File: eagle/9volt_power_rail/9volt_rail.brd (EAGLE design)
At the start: 96.2 x 63.2 mm, 22 parts

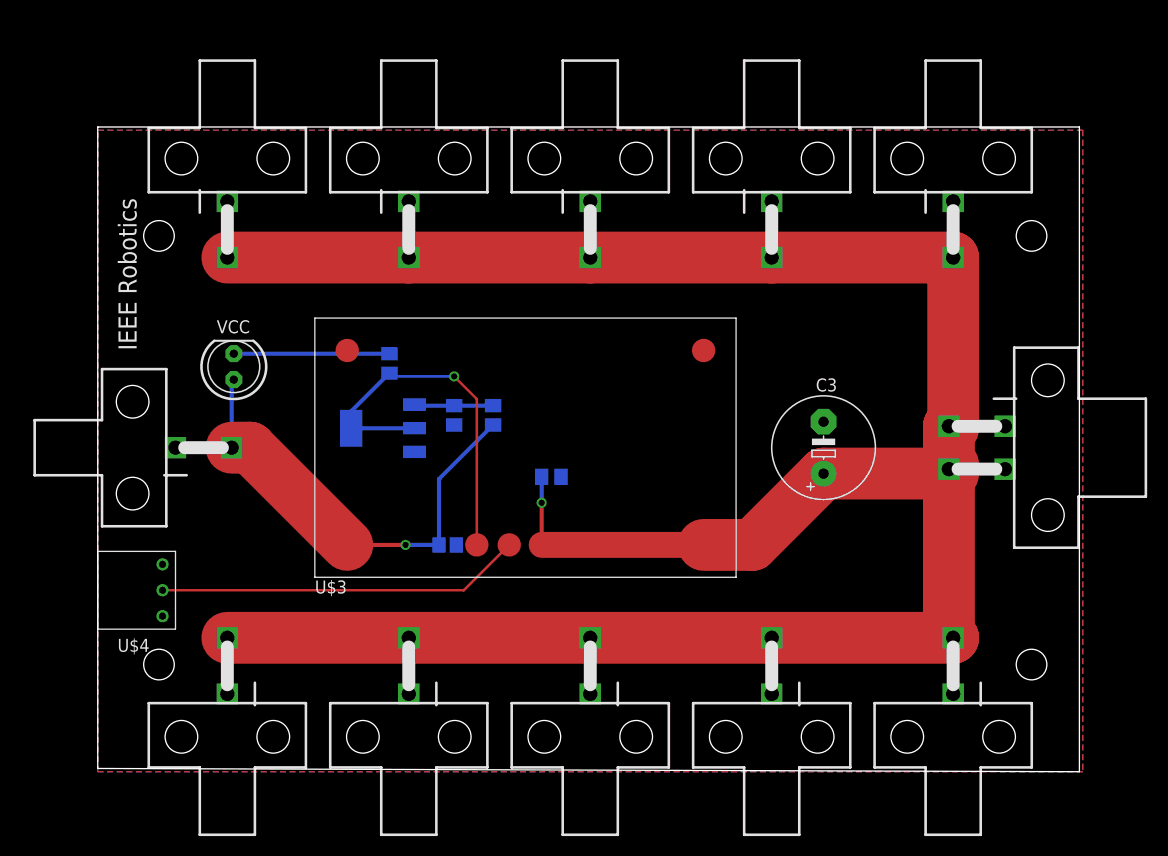
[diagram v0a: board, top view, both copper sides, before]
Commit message: Done with revision B
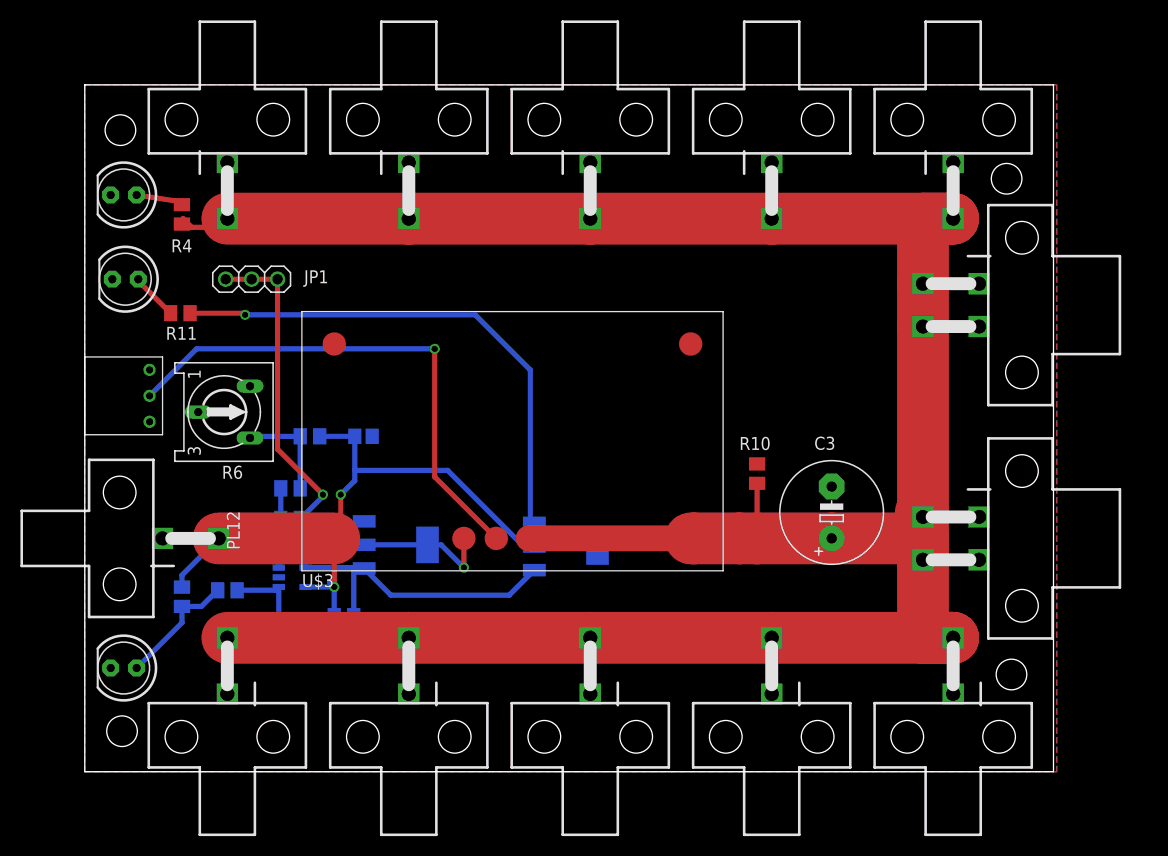
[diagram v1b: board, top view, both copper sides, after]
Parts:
- removed VCC: (no value), adafruit:LED5MM
- added IC1: TL331, linear:DBV-R-PDSO-G5
- added JP1: (no value), adafruit:1X03
- added PL13: (no value), con-molex-2:5569-4
- added R1, R10, R11, R3, R5, R7: (no value), adafruit:M0805
- added R6: (no value), pot:RS3
- added T1: (no value), zetex:SOT223
- added VCC1, VCC2, VCC3: (no value), adafruit:LED5MM
- moved PL6 85.9 mm to (83.8, 7.62), turned to 0 degrees
- moved PL1 71.9 mm to (12.7, 7.62), turned to 0 degrees
- moved PL2 71.9 mm to (30.5, 7.62), turned to 0 degrees
- moved PL5 63.1 mm to (48.3, 59.7), turned to 180 degrees
- moved PL4 59.9 mm to (66.0, 7.62), turned to 0 degrees
- moved PL7 55.0 mm to (83.8, 59.7), turned to 180 degrees
- moved PL8 55.0 mm to (66.0, 59.7), turned to 180 degrees
- moved PL10 52.1 mm to (12.7, 59.7), turned to 180 degrees
- moved PL9 52.1 mm to (30.5, 59.7), turned to 180 degrees
- moved PL3 48.3 mm to (48.3, 7.62), turned to 0 degrees
- moved R4 44.4 mm to (8.26, 54.6), flipped to the top, turned to 90 degrees
- moved R8 24.5 mm to (24.1, 15.2), turned to 0 degrees
- moved U$4 19.1 mm to (5.08, 36.8)
- moved R9 19.0 mm to (18.9, 24.8), turned to 180 degrees
- moved R2 15.6 mm to (18.9, 27.8), turned to 0 degrees
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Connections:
- removed net N$14: R8.2, R9.1, T3.1
- new net N$10: R11.1, T1.3
- new net N$2: IC1.4, JP1.1, JP1.2, JP1.3, R8.1, R9.2, T1.1, T3.1
- new net N$3: R1.2, R5.1, VCC1.A
- new net N$6: R2.1, R3.2, R6.E
- new net N$7: IC1.1, R5.2, R7.1
- new net N$8: R11.2, VCC3.A
- new net N$9: R4.2, VCC2.A
- net GND: now also IC1.2, PL13.1, PL13.2, R10.2, R6.S, R7.2, VCC1.K, VCC2.K, VCC3.K; no longer R4.2, R9.2
- net N$1: now also PL13.3, PL13.4, R10.1
- net N$4: now also IC1.3, R2.2, R9.1; no longer R2.1, VCC.K
- net N$5: no longer R2.2
- net VCC: now also IC1.5, R1.1, R3.1, R8.2, T1.2, T1.4; no longer R8.1, VCC.A
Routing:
- net N$2: track 0.00 -> 65.9 mm, vias 0 -> 1
- net N$10: track 0.00 -> 50.8 mm, vias 0 -> 1
- net VCC: track 45.1 -> 70.9 mm, vias 1 -> 2
- net N$5: track 37.1 -> 13.5 mm
- net N$12: track 35.8 -> 50.9 mm, vias 0 -> 1
- net N$1: track 231.4 -> 244.8 mm, vias 1 -> 0
- net N$3: track 0.00 -> 12.0 mm
- net N$6: track 0.00 -> 10.1 mm
- net N$7: track 0.00 -> 8.50 mm
- net N$14: track 7.73 -> 0.00 mm
- net N$4: track 15.2 -> 7.84 mm
- net N$8: track 0.00 -> 4.65 mm
- net N$9: track 0.00 -> 4.63 mm
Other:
- board size 96.2 x 63.2 mm -> 94.9 x 67.3 mm
- board text removed: "IEEE Robotics"
